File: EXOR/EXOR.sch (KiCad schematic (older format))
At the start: 4 parts

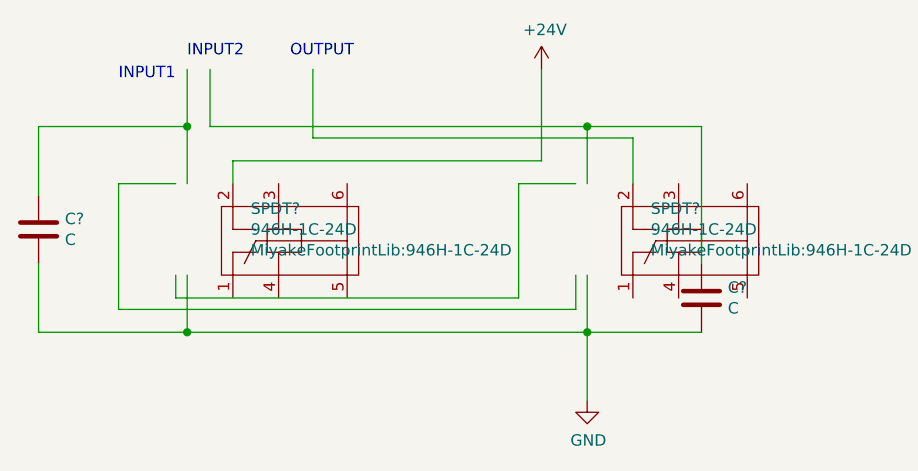
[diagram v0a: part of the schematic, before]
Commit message: Add files via upload
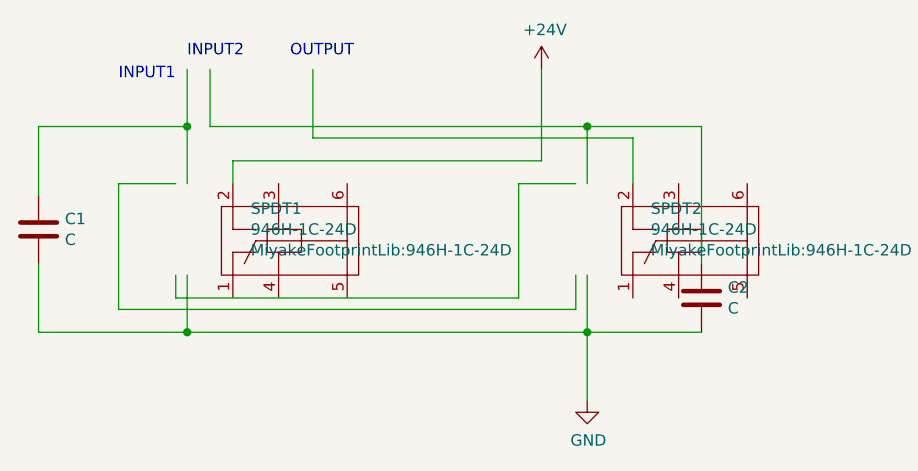
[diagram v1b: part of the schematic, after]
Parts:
- gave numbers to parts that had none: 4
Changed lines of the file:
@@
 $EndDescr
 $Comp
-L MiyakeLib:946H-1C-24D SPDT?
+L MiyakeLib:946H-1C-24D SPDT1
 U 1 1 5ED09565
 P 3400 2600
-F 0 "SPDT?" V 3491 2372 50  0000 R CNN
+F 0 "SPDT1" V 3491 2372 50  0000 R CNN
 F 1 "946H-1C-24D" V 3400 2372 50  0000 R CNN
 F 2 "MiyakeFootprintLib:946H-1C-24D" V 3309 2372 50  0000 R CNN
@@
 $EndComp
 $Comp
-L MiyakeLib:946H-1C-24D SPDT?
+L MiyakeLib:946H-1C-24D SPDT2
 U 1 1 5ED09F1B
 P 5150 2600
-F 0 "SPDT?" V 5241 2372 50  0000 R CNN
+F 0 "SPDT2" V 5241 2372 50  0000 R CNN
 F 1 "946H-1C-24D" V 5150 2372 50  0000 R CNN
 F 2 "MiyakeFootprintLib:946H-1C-24D" V 5059 2372 50  0000 R CNN
@@
 OUTPUT
 $Comp
-L power:+24V #PWR?
+L power:+24V #PWR01
 U 1 1 5ED0D7F2
 P 4900 1900
-F 0 "#PWR?" H 4900 1750 50  0001 C CNN
+F 0 "#PWR01" H 4900 1750 50  0001 C CNN
 F 1 "+24V" H 4915 2073 50  0000 C CNN
 F 2 "" H 4900 1900 50  0001 C CNN
@@
 $EndComp
 $Comp
-L power:GND #PWR?
+L power:GND #PWR02
 U 1 1 5ED0E393
 P 5100 3350
-F 0 "#PWR?" H 5100 3100 50  0001 C CNN
+F 0 "#PWR02" H 5100 3100 50  0001 C CNN
 F 1 "GND" H 5105 3177 50  0000 C CNN
 F 2 "" H 5100 3350 50  0001 C CNN
@@
 $EndComp
 $Comp
-L Device:C C?
+L Device:C C1
 U 1 1 5ED1E6B5
 P 2700 2600
-F 0 "C?" H 2815 2646 50  0000 L CNN
+F 0 "C1" H 2815 2646 50  0000 L CNN
 F 1 "C" H 2815 2555 50  0000 L CNN
 F 2 "" H 2738 2450 50  0001 C CNN
@@
 $EndComp
 $Comp
-L Device:C C?
+L Device:C C2
 U 1 1 5ED1FB24
 P 5600 2900
-F 0 "C?" H 5715 2946 50  0000 L CNN
+F 0 "C2" H 5715 2946 50  0000 L CNN
 F 1 "C" H 5715 2855 50  0000 L CNN
 F 2 "" H 5638 2750 50  0001 C CNN

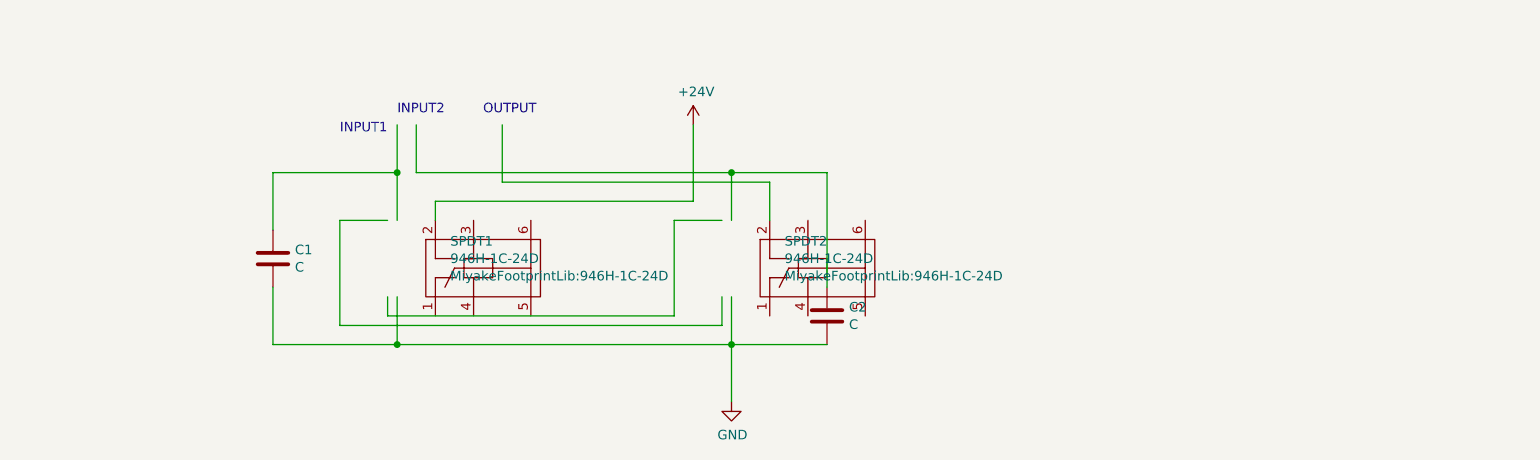
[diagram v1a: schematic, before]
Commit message: Add files via upload
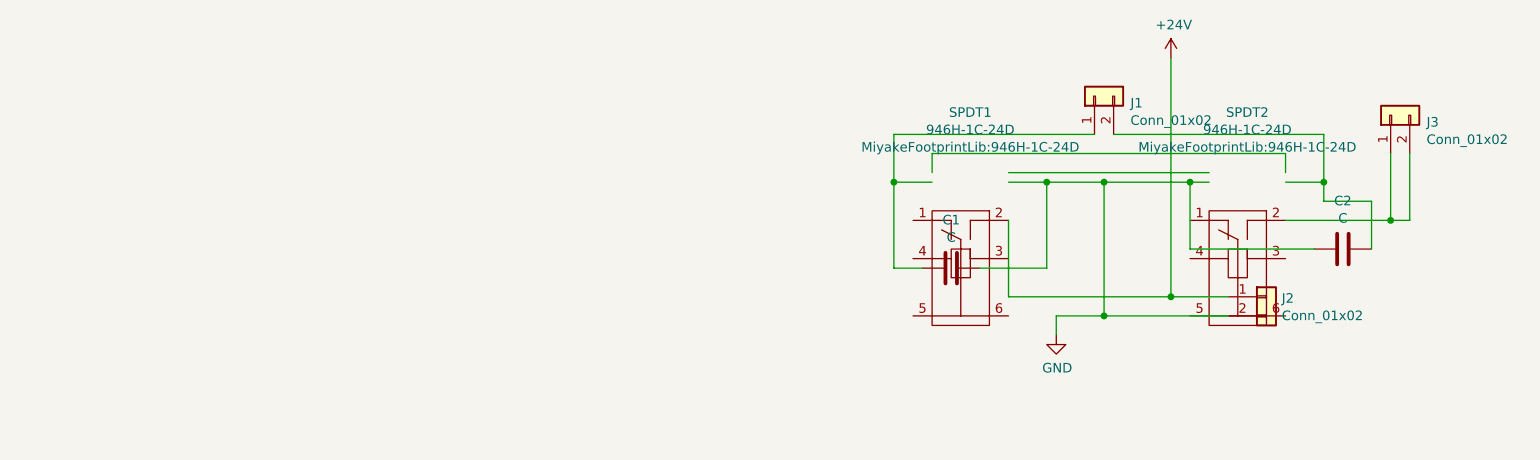
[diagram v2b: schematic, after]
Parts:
- added J1, J2, J3: Conn_01x02, Connector_PinHeader_2.54mm:PinHeader_1x02_P2.54mm_Vertical, symbol Connector_Generic:Conn_01x02
- C1, C2: footprint (none) -> MiyakeFootprintLib:Condensor
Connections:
- wire segments 30 -> 35
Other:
- note removed: "INPUT1"
- note removed: "INPUT2"
- note removed: "OUTPUT"
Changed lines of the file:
@@
 $Comp
 L MiyakeLib:946H-1C-24D SPDT1
-U 1 1 5ED09565
-P 3400 2600
-F 0 "SPDT1" V 3491 2372 50  0000 R CNN
-F 1 "946H-1C-24D" V 3400 2372 50  0000 R CNN
-F 2 "MiyakeFootprintLib:946H-1C-24D" V 3309 2372 50  0000 R CNN
-F 3 "" H 3350 2850 50  0001 C CNN
-	1    3400 2600
-	0    -1   -1   0
+U 1 1 5ED5344E
+P 6350 2250
+F 0 "SPDT1" H 6350 2665 50  0000 C CNN
+F 1 "946H-1C-24D" H 6350 2574 50  0000 C CNN
+F 2 "MiyakeFootprintLib:946H-1C-24D" H 6350 2483 50  0000 C CNN
+F 3 "" H 6300 2500 50  0001 C CNN
+	1    6350 2250
+	1    0    0    -1
 $EndComp
 $Comp
 L MiyakeLib:946H-1C-24D SPDT2
-U 1 1 5ED09F1B
-P 5150 2600
-F 0 "SPDT2" V 5241 2372 50  0000 R CNN
-F 1 "946H-1C-24D" V 5150 2372 50  0000 R CNN
-F 2 "MiyakeFootprintLib:946H-1C-24D" V 5059 2372 50  0000 R CNN
-F 3 "" H 5100 2850 50  0001 C CNN
-	1    5150 2600
+U 1 1 5ED53C3E
+P 7800 2250
+F 0 "SPDT2" H 7800 2665 50  0000 C CNN
+F 1 "946H-1C-24D" H 7800 2574 50  0000 C CNN
+F 2 "MiyakeFootprintLib:946H-1C-24D" H 7800 2483 50  0000 C CNN
+F 3 "" H 7750 2500 50  0001 C CNN
+	1    7800 2250
+	1    0    0    -1
+$EndComp
+$Comp
+L Connector_Generic:Conn_01x02 J1
+U 1 1 5ED54E87
+P 7000 1750
+F 0 "J1" V 6964 1562 50  0000 R CNN
+F 1 "Conn_01x02" V 6873 1562 50  0000 R CNN
+F 2 "Connector_PinHeader_2.54mm:PinHeader_1x02_P2.54mm_Vertical" H 7000 1750 50  0001 C CNN
+F 3 "~" H 7000 1750 50  0001 C CNN
+	1    7000 1750
 	0    -1   -1   0
 $EndComp
 Wire Wire Line
-	3350 2400 3350 2150
+	7000 1950 5950 1950
 Wire Wire Line
-	5100 2400 5100 2150
+	5950 1950 5950 2200
 Wire Wire Line
-	5100 2150 3450 2150
+	5950 2200 6150 2200
 Wire Wire Line
-	3450 2150 3450 1900
+	7100 1950 8200 1950
 Wire Wire Line
-	3350 2800 3350 3050
+	8200 1950 8200 2200
 Wire Wire Line
-	3350 3050 5100 3050
+	8200 2200 8000 2200
 Wire Wire Line
-	5100 3050 5100 2800
-Connection ~ 5100 3050
+	6550 2200 6750 2200
 Wire Wire Line
-	5100 3050 5100 3350
+	7050 2900 6800 2900
 Wire Wire Line
-	3550 2400 3550 2300
+	6800 2900 6800 3000
 Wire Wire Line
-	3550 2300 4900 2300
+	7050 2200 7050 2900
+Connection ~ 7050 2200
 Wire Wire Line
-	4900 2300 4900 1900
+	7050 2200 7500 2200
+$Comp
+L power:GND #PWR01
+U 1 1 5ED55E00
+P 6800 3000
+F 0 "#PWR01" H 6800 2750 50  0001 C CNN
+F 1 "GND" H 6805 2827 50  0000 C CNN
+F 2 "" H 6800 3000 50  0001 C CNN
+F 3 "" H 6800 3000 50  0001 C CNN
+	1    6800 3000
+	1    0    0    -1
+$EndComp
 Wire Wire Line
-	5300 2400 5300 2200
+	7050 2900 7700 2900
+Connection ~ 7050 2900
+$Comp
+L Connector_Generic:Conn_01x02 J2
+U 1 1 5ED565F3
+P 7900 2800
+F 0 "J2" H 7980 2792 50  0000 L CNN
+F 1 "Conn_01x02" H 7980 2701 50  0000 L CNN
+F 2 "Connector_PinHeader_2.54mm:PinHeader_1x02_P2.54mm_Vertical" H 7900 2800 50  0001 C CNN
+F 3 "~" H 7900 2800 50  0001 C CNN
+	1    7900 2800
+	1    0    0    -1
+$EndComp
 Wire Wire Line
-	5300 2200 3900 2200
+	7600 2150 6550 2150
 Wire Wire Line
-	3900 2200 3900 1900
+	6150 2150 6150 2050
 Wire Wire Line
-	3300 2400 3050 2400
+	6150 2050 8000 2050
 Wire Wire Line
-	3050 2400 3050 2950
+	8000 2050 8000 2150
 Wire Wire Line
-	3050 2950 5050 2950
+	6550 2400 6550 2800
 Wire Wire Line
-	5050 2950 5050 2800
+	6550 2800 7400 2800
 Wire Wire Line
-	3300 2800 3300 2900
+	7400 2800 7400 1550
+Connection ~ 7400 2800
 Wire Wire Line
-	3300 2900 4800 2900
-Wire Wire Line
-	4800 2900 4800 2400
-Wire Wire Line
-	4800 2400 5050 2400
-Text Notes 3050 1950 0    50   ~ 0
-INPUT1
-Text Notes 3350 1850 0    50   ~ 0
-INPUT2
-Text Notes 3800 1850 0    50   ~ 0
-OUTPUT
+	7400 2800 7700 2800
 $Comp
-L power:+24V #PWR01
-U 1 1 5ED0D7F2
-P 4900 1900
-F 0 "#PWR01" H 4900 1750 50  0001 C CNN
-F 1 "+24V" H 4915 2073 50  0000 C CNN
-F 2 "" H 4900 1900 50  0001 C CNN
-F 3 "" H 4900 1900 50  0001 C CNN
-	1    4900 1900
+L power:+24V #PWR02
+U 1 1 5ED57508
+P 7400 1550
+F 0 "#PWR02" H 7400 1400 50  0001 C CNN
+F 1 "+24V" H 7415 1723 50  0000 C CNN
+F 2 "" H 7400 1550 50  0001 C CNN
+F 3 "" H 7400 1550 50  0001 C CNN
+	1    7400 1550
 	1    0    0    -1
 $EndComp
 $Comp
-L power:GND #PWR02
-U 1 1 5ED0E393
-P 5100 3350
-F 0 "#PWR02" H 5100 3100 50  0001 C CNN
-F 1 "GND" H 5105 3177 50  0000 C CNN
-F 2 "" H 5100 3350 50  0001 C CNN
-F 3 "" H 5100 3350 50  0001 C CNN
-	1    5100 3350
-	1    0    0    -1
+L Connector_Generic:Conn_01x02 J3
+U 1 1 5ED577C2
+P 8550 1850
+F 0 "J3" V 8514 1662 50  0000 R CNN
+F 1 "Conn_01x02" V 8423 1662 50  0000 R CNN
+F 2 "Connector_PinHeader_2.54mm:PinHeader_1x02_P2.54mm_Vertical" H 8550 1850 50  0001 C CNN
+F 3 "~" H 8550 1850 50  0001 C CNN
+	1    8550 1850
+	0    -1   -1   0
 $EndComp
+Wire Wire Line
+	8000 2400 8550 2400
+Wire Wire Line
+	8550 2400 8550 2050
+Wire Wire Line
+	8650 2050 8650 2400
+Wire Wire Line
+	8650 2400 8550 2400
+Connection ~ 8550 2400
+$Comp
+L Device:C C2
+U 1 1 5ED58715
+P 8300 2550
+F 0 "C2" V 8048 2550 50  0000 C CNN
+F 1 "C" V 8139 2550 50  0000 C CNN
+F 2 "MiyakeFootprintLib:Condensor" H 8338 2400 50  0001 C CNN
+F 3 "~" H 8300 2550 50  0001 C CNN
+	1    8300 2550
+	0    1    1    0
+$EndComp
+Wire Wire Line
+	8200 2200 8200 2300
+Wire Wire Line
+	8200 2300 8450 2300
+Wire Wire Line
+	8450 2300 8450 2550
+Connection ~ 8200 2200
+Wire Wire Line
+	8150 2550 7500 2550
+Wire Wire Line
+	7500 2550 7500 2200
+Connection ~ 7500 2200
+Wire Wire Line
+	7500 2200 7600 2200
 $Comp
 L Device:C C1
-U 1 1 5ED1E6B5
-P 2700 2600
-F 0 "C1" H 2815 2646 50  0000 L CNN
-F 1 "C" H 2815 2555 50  0000 L CNN
-F 2 "" H 2738 2450 50  0001 C CNN
-F 3 "~" H 2700 2600 50  0001 C CNN
-	1    2700 2600
-	1    0    0    -1
-$EndComp
-$Comp
-L Device:C C2
-U 1 1 5ED1FB24
-P 5600 2900
-F 0 "C2" H 5715 2946 50  0000 L CNN
-F 1 "C" H 5715 2855 50  0000 L CNN
-F 2 "" H 5638 2750 50  0001 C CNN
-F 3 "~" H 5600 2900 50  0001 C CNN
-	1    5600 2900
-	1    0    0    -1
+U 1 1 5ED5941C
+P 6250 2650
+F 0 "C1" V 5998 2650 50  0000 C CNN
+F 1 "C" V 6089 2650 50  0000 C CNN
+F 2 "MiyakeFootprintLib:Condensor" H 6288 2500 50  0001 C CNN
+F 3 "~" H 6250 2650 50  0001 C CNN
+	1    6250 2650
+	0    1    1    0
 $EndComp
 Wire Wire Line
-	2700 2450 2700 2150
+	6400 2650 6750 2650
 Wire Wire Line
-	2700 2150 3350 2150
-Connection ~ 3350 2150
+	6750 2650 6750 2200
+Connection ~ 6750 2200
 Wire Wire Line
-	3350 2150 3350 1900
+	6750 2200 7050 2200
 Wire Wire Line
-	2700 2750 2700 3050
+	6100 2650 5950 2650
 Wire Wire Line
-	2700 3050 3350 3050
-Connection ~ 3350 3050
-Wire Wire Line
-	5600 2750 5600 2150
-Wire Wire Line
-	5600 2150 5100 2150
-Connection ~ 5100 2150
-Wire Wire Line
-	5600 3050 5100 3050
+	5950 2650 5950 2200
+Connection ~ 5950 2200
 $EndSCHEMATC

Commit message: Add files via upload
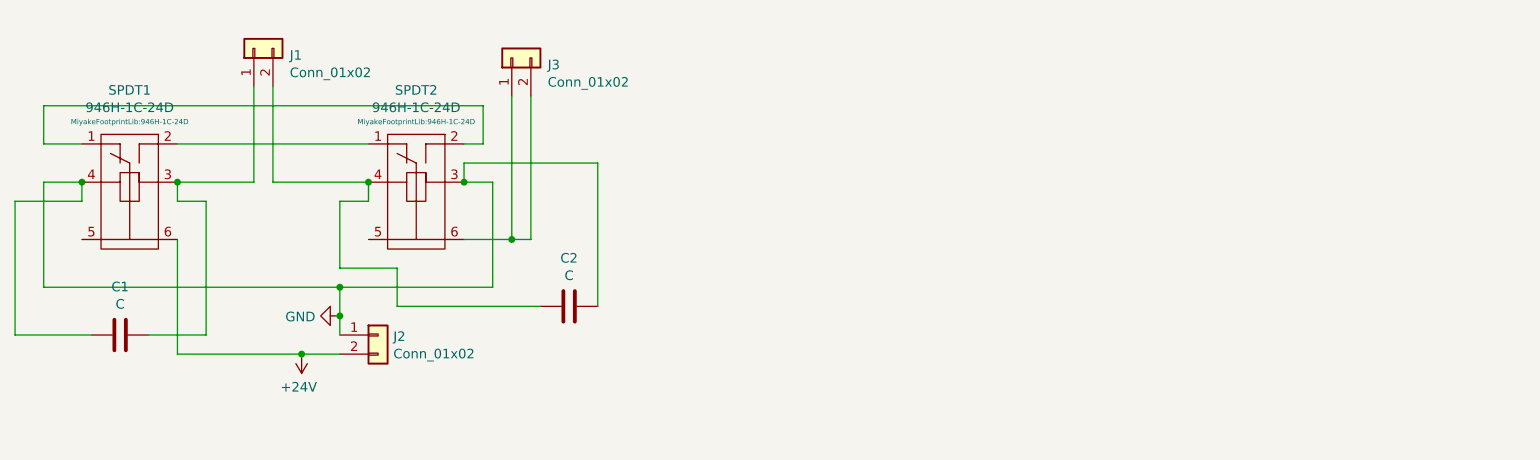
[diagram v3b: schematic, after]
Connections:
- wire segments 35 -> 42
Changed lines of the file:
@@
 $Comp
 L MiyakeLib:946H-1C-24D SPDT1
-U 1 1 5ED5344E
-P 6350 2250
-F 0 "SPDT1" H 6350 2665 50  0000 C CNN
-F 1 "946H-1C-24D" H 6350 2574 50  0000 C CNN
-F 2 "MiyakeFootprintLib:946H-1C-24D" H 6350 2483 50  0000 C CNN
-F 3 "" H 6300 2500 50  0001 C CNN
-	1    6350 2250
+U 1 1 5ED7F418
+P 2000 1850
+F 0 "SPDT1" H 1950 1981 50  0000 C CNN
+F 1 "946H-1C-24D" H 1950 1890 50  0000 C CNN
+F 2 "MiyakeFootprintLib:946H-1C-24D" H 1950 1816 27  0000 C CNN
+F 3 "" V 1950 1300 50  0001 C CNN
+	1    2000 1850
 	1    0    0    -1
 $EndComp
 $Comp
 L MiyakeLib:946H-1C-24D SPDT2
-U 1 1 5ED53C3E
-P 7800 2250
-F 0 "SPDT2" H 7800 2665 50  0000 C CNN
-F 1 "946H-1C-24D" H 7800 2574 50  0000 C CNN
-F 2 "MiyakeFootprintLib:946H-1C-24D" H 7800 2483 50  0000 C CNN
-F 3 "" H 7750 2500 50  0001 C CNN
-	1    7800 2250
+U 1 1 5ED7FB89
+P 3500 1850
+F 0 "SPDT2" H 3450 1981 50  0000 C CNN
+F 1 "946H-1C-24D" H 3450 1890 50  0000 C CNN
+F 2 "MiyakeFootprintLib:946H-1C-24D" H 3450 1816 27  0000 C CNN
+F 3 "" V 3450 1300 50  0001 C CNN
+	1    3500 1850
 	1    0    0    -1
 $EndComp
 $Comp
 L Connector_Generic:Conn_01x02 J1
-U 1 1 5ED54E87
-P 7000 1750
-F 0 "J1" V 6964 1562 50  0000 R CNN
-F 1 "Conn_01x02" V 6873 1562 50  0000 R CNN
-F 2 "Connector_PinHeader_2.54mm:PinHeader_1x02_P2.54mm_Vertical" H 7000 1750 50  0001 C CNN
-F 3 "~" H 7000 1750 50  0001 C CNN
-	1    7000 1750
+U 1 1 5ED80B9E
+P 2600 1500
+F 0 "J1" V 2564 1312 50  0000 R CNN
+F 1 "Conn_01x02" V 2473 1312 50  0000 R CNN
+F 2 "Connector_PinHeader_2.54mm:PinHeader_1x02_P2.54mm_Vertical" H 2600 1500 50  0001 C CNN
+F 3 "~" H 2600 1500 50  0001 C CNN
+	1    2600 1500
 	0    -1   -1   0
 $EndComp
 Wire Wire Line
-	7000 1950 5950 1950
+	2200 2200 2600 2200
 Wire Wire Line
-	5950 1950 5950 2200
+	2600 2200 2600 1700
 Wire Wire Line
-	5950 2200 6150 2200
+	3200 2200 2700 2200
 Wire Wire Line
-	7100 1950 8200 1950
+	2700 2200 2700 1700
+$Comp
+L Connector_Generic:Conn_01x02 J3
+U 1 1 5ED8157C
+P 3950 1550
+F 0 "J3" V 3914 1362 50  0000 R CNN
+F 1 "Conn_01x02" V 3823 1362 50  0000 R CNN
+F 2 "Connector_PinHeader_2.54mm:PinHeader_1x02_P2.54mm_Vertical" H 3950 1550 50  0001 C CNN
+F 3 "~" H 3950 1550 50  0001 C CNN
+	1    3950 1550
+	0    -1   -1   0
+$EndComp
 Wire Wire Line
-	8200 1950 8200 2200
+	3700 2500 3950 2500
 Wire Wire Line
-	8200 2200 8000 2200
+	3950 2500 3950 1750
 Wire Wire Line
-	6550 2200 6750 2200
+	3950 2500 4050 2500
 Wire Wire Line
-	7050 2900 6800 2900
-Wire Wire Line
-	6800 2900 6800 3000
-Wire Wire Line
-	7050 2200 7050 2900
-Connection ~ 7050 2200
-Wire Wire Line
-	7050 2200 7500 2200
+	4050 2500 4050 1750
+Connection ~ 3950 2500
 $Comp
-L power:GND #PWR01
-U 1 1 5ED55E00
-P 6800 3000
-F 0 "#PWR01" H 6800 2750 50  0001 C CNN
-F 1 "GND" H 6805 2827 50  0000 C CNN
-F 2 "" H 6800 3000 50  0001 C CNN
-F 3 "" H 6800 3000 50  0001 C CNN
-	1    6800 3000
+L Connector_Generic:Conn_01x02 J2
+U 1 1 5ED81F9D
+P 3250 3000
+F 0 "J2" H 3330 2992 50  0000 L CNN
+F 1 "Conn_01x02" H 3330 2901 50  0000 L CNN
+F 2 "Connector_PinHeader_2.54mm:PinHeader_1x02_P2.54mm_Vertical" H 3250 3000 50  0001 C CNN
+F 3 "~" H 3250 3000 50  0001 C CNN
+	1    3250 3000
 	1    0    0    -1
 $EndComp
 Wire Wire Line
-	7050 2900 7700 2900
-Connection ~ 7050 2900
+	2200 2500 2200 3100
+Wire Wire Line
+	2200 3100 2850 3100
+Wire Wire Line
+	3700 2200 3850 2200
+Wire Wire Line
+	3850 2200 3850 2750
+Wire Wire Line
+	3850 2750 3050 2750
+Wire Wire Line
+	1500 2750 1500 2200
+Wire Wire Line
+	1500 2200 1700 2200
+Wire Wire Line
+	3050 2750 3050 2900
+Connection ~ 3050 2750
+Wire Wire Line
+	3050 2750 1500 2750
+Wire Wire Line
+	2200 2000 3200 2000
+Wire Wire Line
+	1700 2000 1500 2000
+Wire Wire Line
+	1500 2000 1500 1800
+Wire Wire Line
+	1500 1800 3800 1800
+Wire Wire Line
+	3800 1800 3800 2000
+Wire Wire Line
+	3800 2000 3700 2000
 $Comp
-L Connector_Generic:Conn_01x02 J2
-U 1 1 5ED565F3
-P 7900 2800
-F 0 "J2" H 7980 2792 50  0000 L CNN
-F 1 "Conn_01x02" H 7980 2701 50  0000 L CNN
-F 2 "Connector_PinHeader_2.54mm:PinHeader_1x02_P2.54mm_Vertical" H 7900 2800 50  0001 C CNN
-F 3 "~" H 7900 2800 50  0001 C CNN
-	1    7900 2800
-	1    0    0    -1
-$EndComp
-Wire Wire Line
-	7600 2150 6550 2150
-Wire Wire Line
-	6150 2150 6150 2050
-Wire Wire Line
-	6150 2050 8000 2050
-Wire Wire Line
-	8000 2050 8000 2150
-Wire Wire Line
-	6550 2400 6550 2800
-Wire Wire Line
-	6550 2800 7400 2800
-Wire Wire Line
-	7400 2800 7400 1550
-Connection ~ 7400 2800
-Wire Wire Line
-	7400 2800 7700 2800
-$Comp
-L power:+24V #PWR02
-U 1 1 5ED57508
-P 7400 1550
-F 0 "#PWR02" H 7400 1400 50  0001 C CNN
-F 1 "+24V" H 7415 1723 50  0000 C CNN
-F 2 "" H 7400 1550 50  0001 C CNN
-F 3 "" H 7400 1550 50  0001 C CNN
-	1    7400 1550
-	1    0    0    -1
+L Device:C C2
+U 1 1 5ED83852
+P 4250 2850
+F 0 "C2" V 3998 2850 50  0000 C CNN
+F 1 "C" V 4089 2850 50  0000 C CNN
+F 2 "MiyakeFootprintLib:Condensor" H 4288 2700 50  0001 C CNN
+F 3 "~" H 4250 2850 50  0001 C CNN
+	1    4250 2850
+	0    1    1    0
 $EndComp
 $Comp
-L Connector_Generic:Conn_01x02 J3
-U 1 1 5ED577C2
-P 8550 1850
-F 0 "J3" V 8514 1662 50  0000 R CNN
-F 1 "Conn_01x02" V 8423 1662 50  0000 R CNN
-F 2 "Connector_PinHeader_2.54mm:PinHeader_1x02_P2.54mm_Vertical" H 8550 1850 50  0001 C CNN
-F 3 "~" H 8550 1850 50  0001 C CNN
-	1    8550 1850
-	0    -1   -1   0
-$EndComp
-Wire Wire Line
-	8000 2400 8550 2400
-Wire Wire Line
-	8550 2400 8550 2050
-Wire Wire Line
-	8650 2050 8650 2400
-Wire Wire Line
-	8650 2400 8550 2400
-Connection ~ 8550 2400
-$Comp
-L Device:C C2
-U 1 1 5ED58715
-P 8300 2550
-F 0 "C2" V 8048 2550 50  0000 C CNN
-F 1 "C" V 8139 2550 50  0000 C CNN
-F 2 "MiyakeFootprintLib:Condensor" H 8338 2400 50  0001 C CNN
-F 3 "~" H 8300 2550 50  0001 C CNN
-	1    8300 2550
+L Device:C C1
+U 1 1 5ED83D7D
+P 1900 3000
+F 0 "C1" V 1648 3000 50  0000 C CNN
+F 1 "C" V 1739 3000 50  0000 C CNN
+F 2 "MiyakeFootprintLib:Condensor" H 1938 2850 50  0001 C CNN
+F 3 "~" H 1900 3000 50  0001 C CNN
+	1    1900 3000
 	0    1    1    0
 $EndComp
 Wire Wire Line
-	8200 2200 8200 2300
+	4400 2850 4400 2100
 Wire Wire Line
-	8200 2300 8450 2300
+	4400 2100 3700 2100
 Wire Wire Line
-	8450 2300 8450 2550
-Connection ~ 8200 2200
+	3700 2100 3700 2200
+Connection ~ 3700 2200
 Wire Wire Line
-	8150 2550 7500 2550
+	4100 2850 3350 2850
 Wire Wire Line
-	7500 2550 7500 2200
-Connection ~ 7500 2200
+	3350 2850 3350 2650
 Wire Wire Line
-	7500 2200 7600 2200
+	3350 2650 3050 2650
+Wire Wire Line
+	3050 2650 3050 2300
+Wire Wire Line
+	3050 2300 3200 2300
+Wire Wire Line
+	3200 2300 3200 2200
+Connection ~ 3200 2200
+Wire Wire Line
+	2050 3000 2350 3000
+Wire Wire Line
+	2350 3000 2350 2300
+Wire Wire Line
+	2350 2300 2200 2300
+Wire Wire Line
+	2200 2300 2200 2200
+Connection ~ 2200 2200
+Wire Wire Line
+	1750 3000 1350 3000
+Wire Wire Line
+	1350 3000 1350 2300
+Wire Wire Line
+	1350 2300 1700 2300
+Wire Wire Line
+	1700 2300 1700 2200
+Connection ~ 1700 2200
 $Comp
-L Device:C C1
-U 1 1 5ED5941C
-P 6250 2650
-F 0 "C1" V 5998 2650 50  0000 C CNN
-F 1 "C" V 6089 2650 50  0000 C CNN
-F 2 "MiyakeFootprintLib:Condensor" H 6288 2500 50  0001 C CNN
-F 3 "~" H 6250 2650 50  0001 C CNN
-	1    6250 2650
+L power:GND #PWR?
+U 1 1 5ED89412
+P 3050 2900
+F 0 "#PWR?" H 3050 2650 50  0001 C CNN
+F 1 "GND" V 3055 2772 50  0000 R CNN
+F 2 "" H 3050 2900 50  0001 C CNN
+F 3 "" H 3050 2900 50  0001 C CNN
+	1    3050 2900
 	0    1    1    0
 $EndComp
+Connection ~ 3050 2900
 Wire Wire Line
-	6400 2650 6750 2650
+	3050 2900 3050 3000
+$Comp
+L power:+24V #PWR?
+U 1 1 5ED89782
+P 2850 3100
+F 0 "#PWR?" H 2850 2950 50  0001 C CNN
+F 1 "+24V" H 2865 3273 50  0000 C CNN
+F 2 "" H 2850 3100 50  0001 C CNN
+F 3 "" H 2850 3100 50  0001 C CNN
+	1    2850 3100
+	-1   0    0    1
+$EndComp
+Connection ~ 2850 3100
 Wire Wire Line
-	6750 2650 6750 2200
-Connection ~ 6750 2200
-Wire Wire Line
-	6750 2200 7050 2200
-Wire Wire Line
-	6100 2650 5950 2650
-Wire Wire Line
-	5950 2650 5950 2200
-Connection ~ 5950 2200
+	2850 3100 3050 3100
 $EndSCHEMATC
